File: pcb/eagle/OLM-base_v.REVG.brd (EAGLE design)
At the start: 92.1 x 57.6 mm, 40 parts, among them IC1 ATMEGA, IC2 MCP1702-33, IC3 ENC28J60SP, IC4 DS1307, J1 POWER_JACKPTH, J2 MAGJACK, U1 USD-SOCKETMICRO-SD-SOCKET-TAO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, X1 16 MHz, X2 25MHz, X3 32.657k

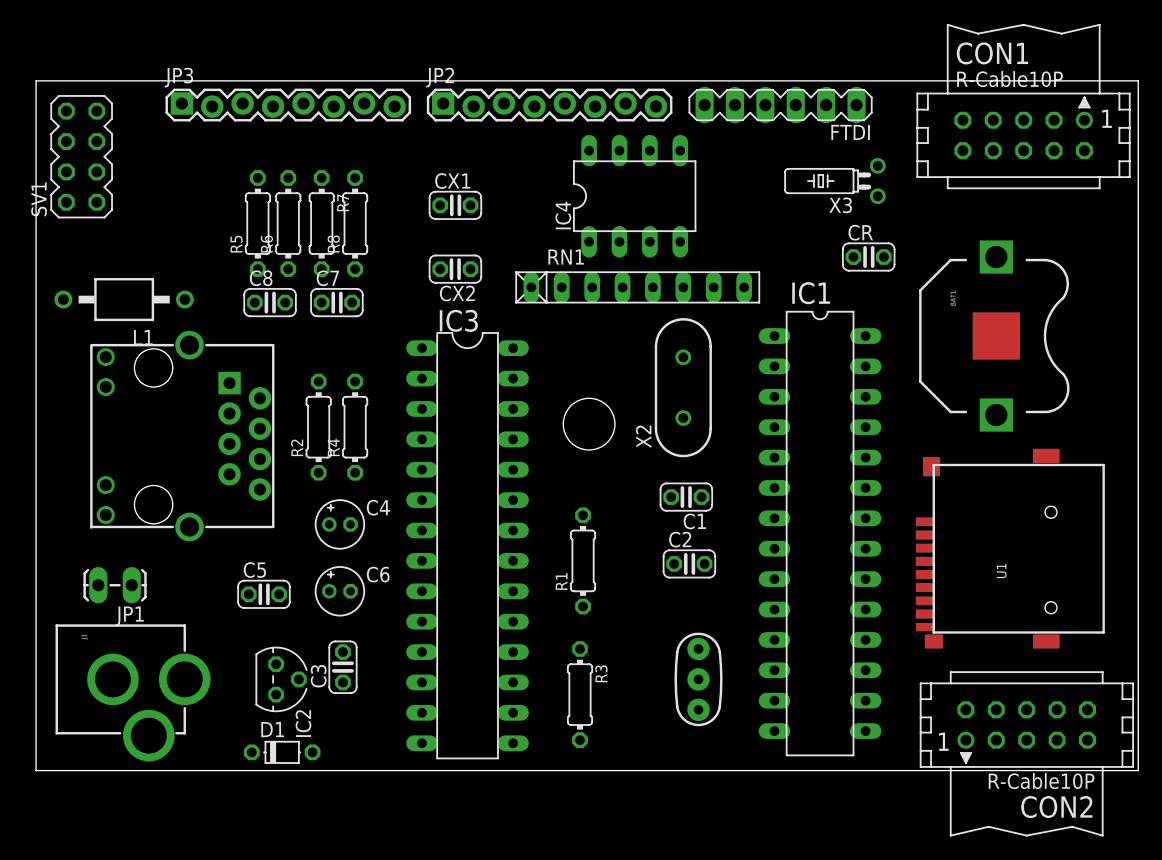
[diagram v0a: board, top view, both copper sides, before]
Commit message: made changes
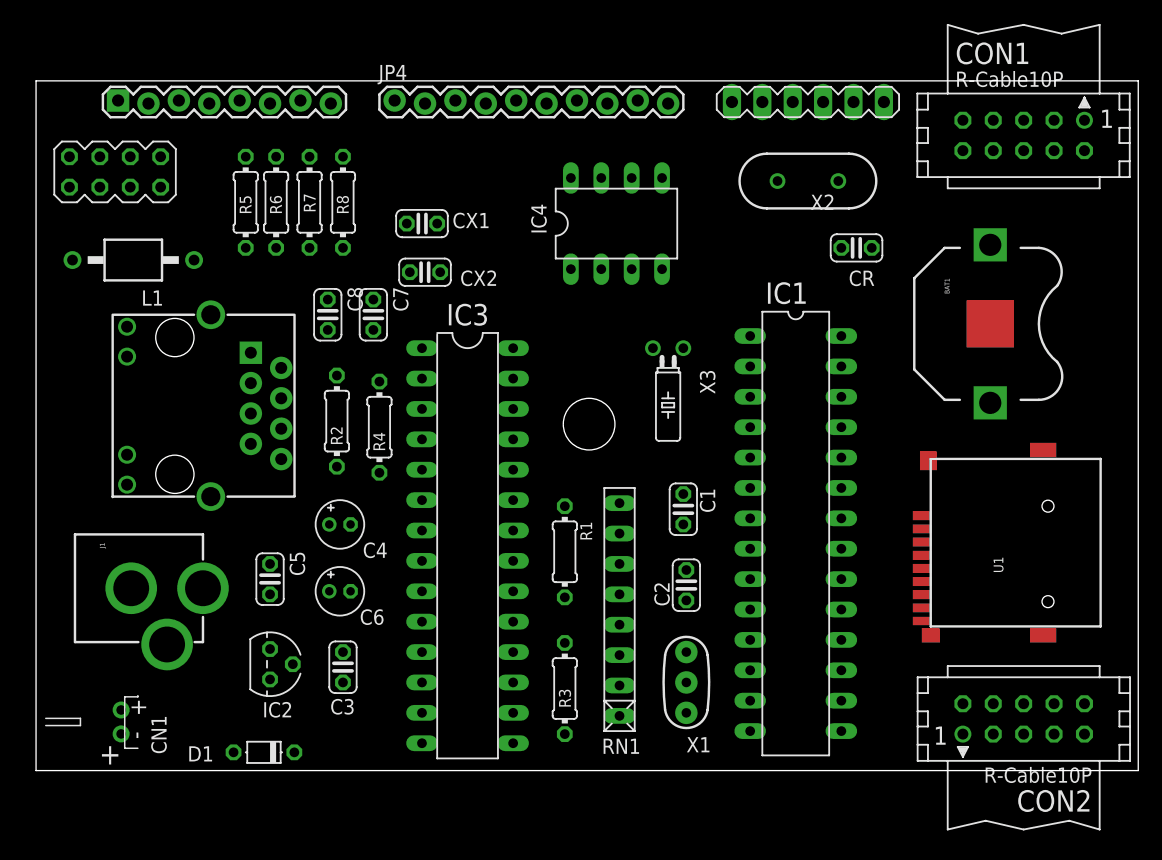
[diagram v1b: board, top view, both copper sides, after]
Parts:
- removed JP1: BATT, SparkFun:1X02_LOCK_LONGPADS
- removed JP2: (no value), SparkFun-Connectors:1X08_LOCK
- added CN1: (no value), adafruit:JST-PH-2-THM-RA
- added JP4: M10LOCK, SparkFun-Connectors:1X10_LOCK
- moved RN1 27.0 mm to (48.8, 13.5), turned to 90 degrees
- moved X3 22.4 mm to (52.8, 35.3), turned to 180 degrees
- moved X2 20.2 mm to (64.5, 49.3), turned to 180 degrees
- moved J1 7.77 mm to (0.25, 15.2)
- moved JP3 5.34 mm to (6.86, 55.9)
- moved C8 4.93 mm to (24.4, 38.1), turned to 90 degrees
- moved L1 3.39 mm to (8.13, 42.7)
- moved C7 3.21 mm to (28.2, 38.1), turned to 90 degrees
- moved CX1 3.18 mm to (32.3, 45.7)
- moved J2 3.10 mm to (0.51, 38.1)
- moved SV1 3.07 mm to (6.60, 50.0), turned to 180 degrees
- moved IC4 2.75 mm to (48.5, 45.7)
- moved CX2 2.55 mm to (32.5, 41.7)
- moved FTDI 2.30 mm to (70.9, 55.9)
- moved R5 2.05 mm to (17.5, 47.5)
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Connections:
- net A4/SDA: now also JP4.10; no longer JP2.8
- net A5/SCL: now also JP4.9; no longer JP2.7
- net D2: now also JP4.3; no longer JP2.4
- net D3/PWM: now also JP4.2; no longer JP2.3
- net D4: now also JP4.6
- net D6/PWM: now also JP4.5
- net D7: now also JP4.4
- net E-CLK: now also JP4.8; no longer JP2.6
- net E-INT: now also JP4.7; no longer JP2.5
- net GND: now also CN1.2, JP4.1; no longer JP1.2, JP2.1
- net MISO/D12: now also U1.7
- net MOSI/D11: now also U1.3
- net SCK/D13: now also U1.5
- net VCC: now also JP3.8; no longer JP2.2
- net VIN: now also CN1.1; no longer JP1.1, JP3.8
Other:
- board text added: "+"
- board text added: "X1"
